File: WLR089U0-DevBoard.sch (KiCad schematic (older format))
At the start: 23 parts, among them IC1 WLR089U0-I_RM, J1 USB_B_Micro, J2 Conn_ARM_JTAG_SWD_10, J3 Conn_01x10_Female, J4 Conn_01x02_Male, J5 Conn_01x10_Female, J6 Conn_01x08_Male, SW1 SW_Push, U1 MCP1700-3302E_SOT23, U2 CH304E

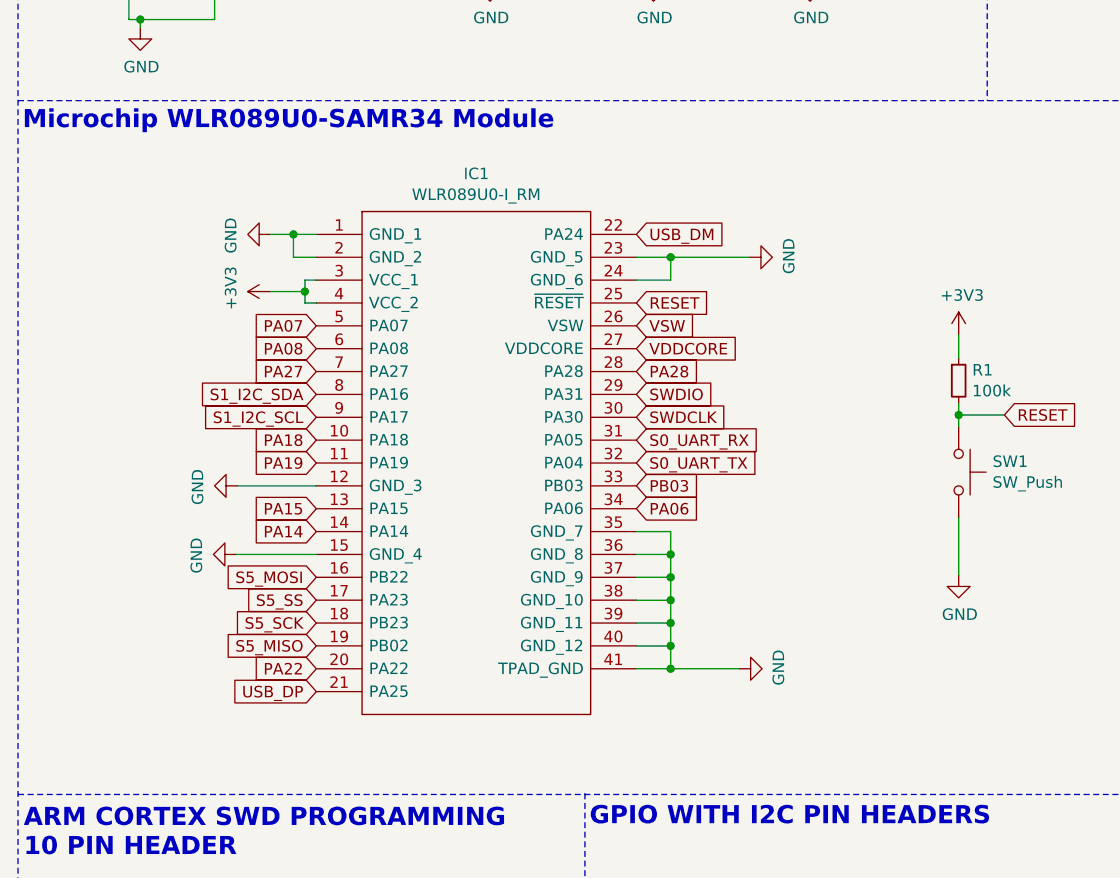
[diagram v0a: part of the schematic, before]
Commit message: editing
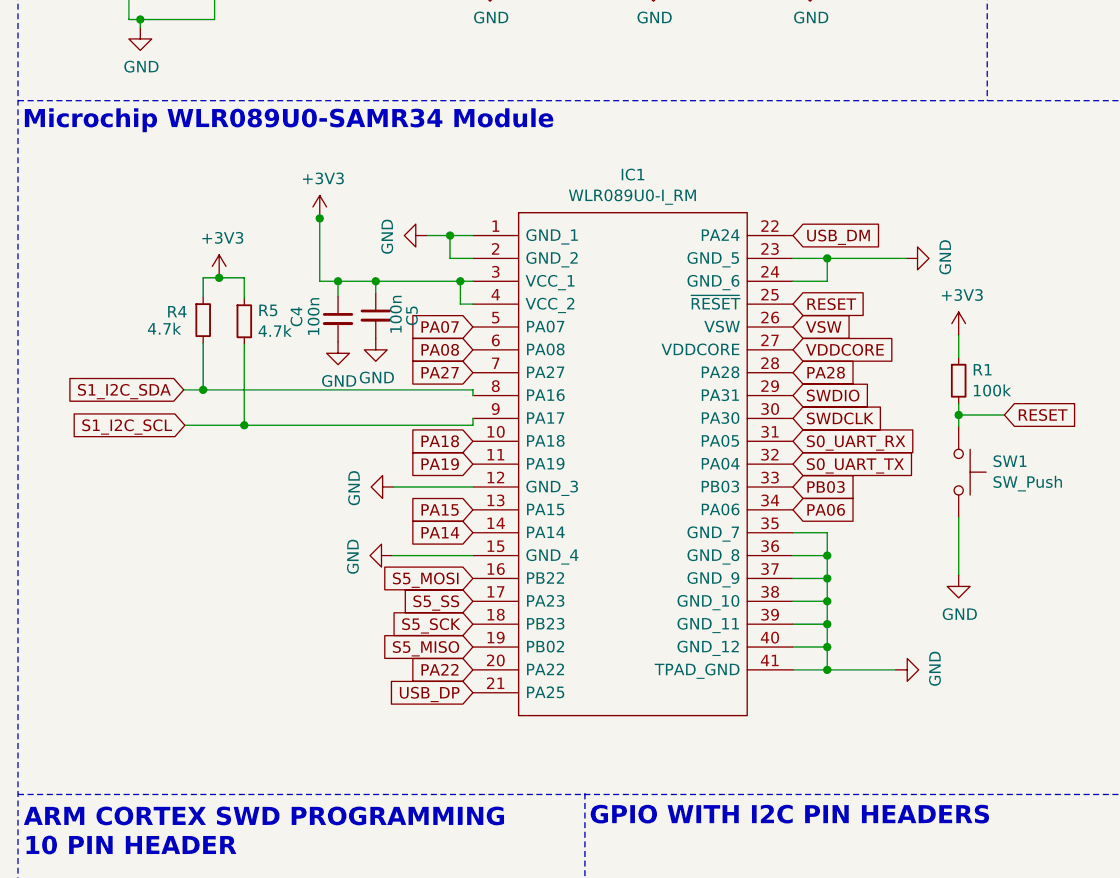
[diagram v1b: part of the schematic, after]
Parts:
- added C4, C5: 100n, Capacitor_SMD:C_0402_1005Metric_Pad0.74x0.62mm_HandSolder, symbol Device:C_Small
- added R4, R5: 4.7k, Resistor_SMD:R_1206_3216Metric_Pad1.42x1.75mm_HandSolder, symbol Device:R_Small
- C3: footprint Capacitor_SMD:C_1206_3216Metric_Pad1.33x1.80mm_HandSolder -> Capacitor_SMD:C_0402_1005Metric_Pad0.74x0.62mm_HandSolder
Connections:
- net +3V3: now also C4.1, C5.1, R4.1, R5.1
- net GND: now also C4.2, C5.2
- net S1_I2C_SCL: now also R5.2
- net S1_I2C_SDA: now also R4.2
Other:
- moved on the sheet: IC1
